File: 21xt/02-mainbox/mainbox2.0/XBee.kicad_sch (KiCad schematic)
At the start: 13 parts, among them IC1 XBP9X-DMUS-011, J3 Conn_01x02, J4 Conn_01x02

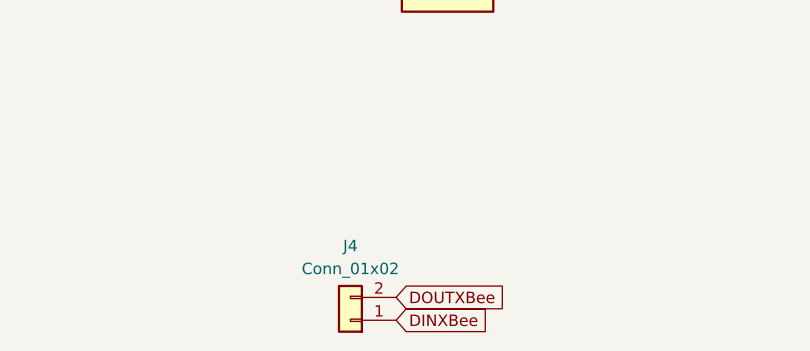
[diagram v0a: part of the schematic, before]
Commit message: sophie needs to fix this
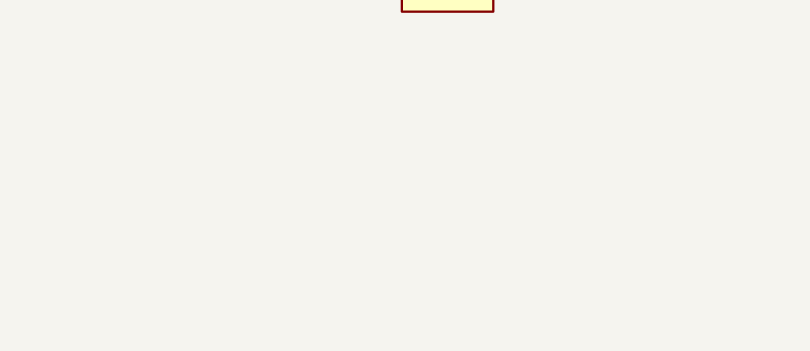
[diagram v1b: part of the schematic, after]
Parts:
- removed J4: Conn_01x02, Connector_PinHeader_2.54mm:PinHeader_1x02_P2.54mm_Vertical, symbol Connector_Generic:Conn_01x02
- PS1: footprint 21xt_footprints:R78B5015L - -> 21xt_footprints:CONV_R-78B3.3-1.5
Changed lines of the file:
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@@
     (effects (font (size 1.27 1.27)) (justify left bottom))
-  )
-  (global_label "DINXBee" (shape input) (at 90.805 143.51 0) (fields_autoplaced)
-    (effects (font (size 1.27 1.27)) (justify left))
-    (property "Intersheetrefs" "${INTERSHEET_REFS}" (at 101.6522 143.51 0)
-      (effects (font (size 1.27 1.27)) (justify left) hide)
-    )
   )
   (global_label "DOUTXBee" (shape output) (at 173.99 71.12 180) (fields_autoplaced)
@@
     )
   )
-  (global_label "DOUTXBee" (shape input) (at 90.805 140.97 0) (fields_autoplaced)
-    (effects (font (size 1.27 1.27)) (justify left))
-    (property "Intersheetrefs" "${INTERSHEET_REFS}" (at 103.3455 140.97 0)
-      (effects (font (size 1.27 1.27)) (justify left) hide)
-    )
-  )
   (symbol (lib_id "power:GND") (at 106.68 81.28 180) (unit 1)
     (in_bom yes) (on_board yes) (dnp no) (fields_autoplaced)
@@
       (effects (font (size 1.27 1.27)) (justify left))
     )
-    (property "Footprint" "21xt_footprints:R78B5015L -" (at 4.14 110.49 0)
+    (property "Footprint" "21xt_footprints:CONV_R-78B3.3-1.5" (at 4.14 110.49 0)
       (effects (font (size 1.27 1.27)) (justify left top) hide)
     )
@@
         )
       )
-    )
-  )
-  (symbol (lib_id "Connector_Generic:Conn_01x02") (at 85.725 143.51 180) (unit 1)
-    (in_bom yes) (on_board yes) (dnp no) (fields_autoplaced)
-    (property "Reference" "J4" (at 85.725 135.255 0)
-      (effects (font (size 1.27 1.27)))
-    )
-    (property "Value" "Conn_01x02" (at 85.725 137.795 0)
-      (effects (font (size 1.27 1.27)))
-    )
-    (property "Footprint" "Connector_PinHeader_2.54mm:PinHeader_1x02_P2.54mm_Vertical" (at 85.725 143.51 0)
-      (effects (font (size 1.27 1.27)) hide)
-    )
-    (property "Datasheet" "~" (at 85.725 143.51 0)
-      (effects (font (size 1.27 1.27)) hide)
-    )
-    (pin "1")
-    (pin "2")
-    (instances
-      (project "mainbox1.0"
-        (path "/386ce652-2291-4cad-85a5-fcca6d2077c3/dd0157a9-838c-4507-b641-fb16517bbb6e"
-          (reference "J4") (unit 1)
-        )
-      )
-      (project "mainbox2.0"
-        (path "/f7ca7218-80bf-4776-ba9d-a28b83375023/5d6e883b-1bc0-4ce9-8a5a-9d01f2a447ea"
-          (reference "J6") (unit 1)
-        )
-      )
-      (project "Mainboard_priv"
-        (path "/fef72a68-b3e4-4609-8f5e-093085beb166/ccbaf9e4-0c9b-47b5-a316-0ae6750baa2c"
-          (reference "J1") (unit 1)
-        )
-      )
